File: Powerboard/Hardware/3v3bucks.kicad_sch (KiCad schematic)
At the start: 26 parts, among them IC2 SiC437AED-T1-GE3, Q5 PXP012-30QLJ, Q6 PXP012-30QLJ, U1 LTC4412xS6, U8 LTC4412xS6

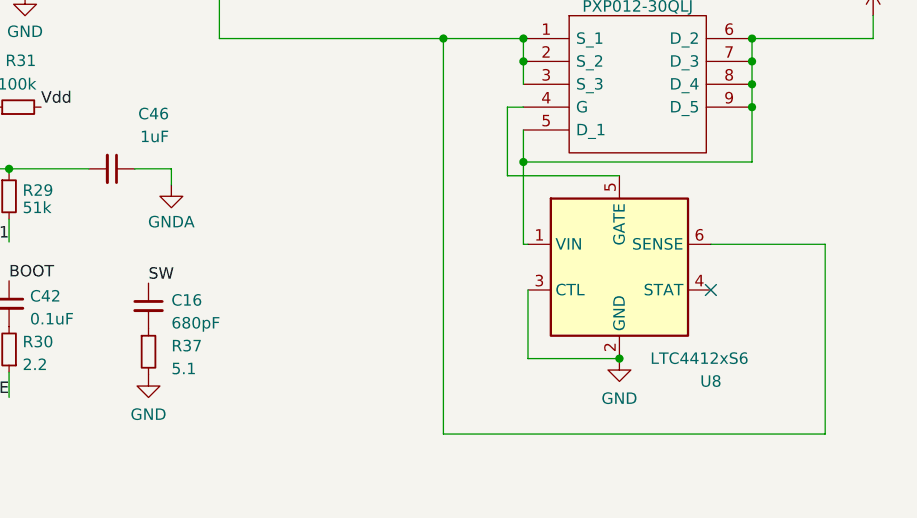
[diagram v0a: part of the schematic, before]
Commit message: post Andrei review
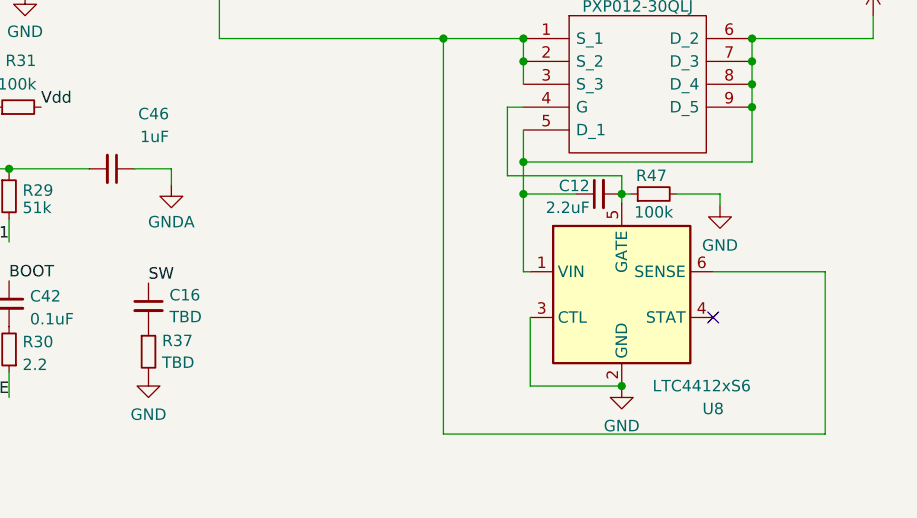
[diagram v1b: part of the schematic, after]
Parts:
- added C12: 2.2uF, Capacitor_SMD:C_0402_1005Metric, symbol Device:C_Small
- added R47: 100k, Resistor_SMD:R_0402_1005Metric, symbol Device:R_Small
- C16: value 680pF -> TBD
- R37: value 5.1 -> TBD
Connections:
- net GND: now also R47.2
- net VBUS: now also C12.1
- net at Q6.4 (G), U8.5 (GATE): now also C12.2, R47.1
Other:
- moved on the sheet: U8
